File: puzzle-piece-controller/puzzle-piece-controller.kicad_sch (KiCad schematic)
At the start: 12 parts, among them J1 POGO PINS, J2 OUTPUT, J3 3.3V, J4 GND, J5 ANALOG, U1 MOUDLE-SEEEDUINO-XIAO-ESP32C3

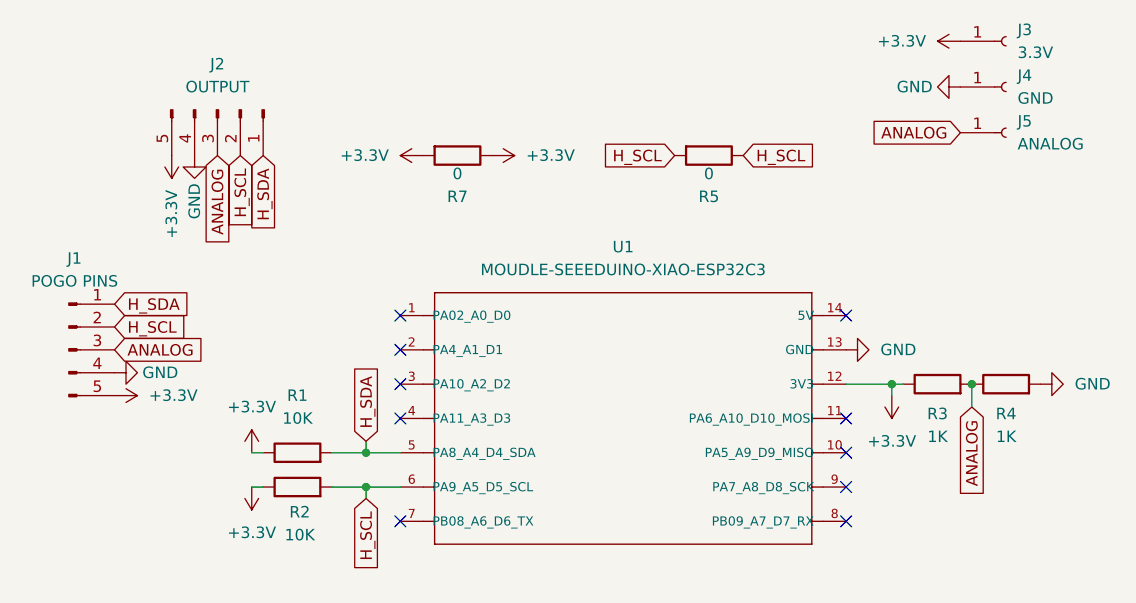
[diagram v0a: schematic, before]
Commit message: current puzzle with attiny and pogo pins
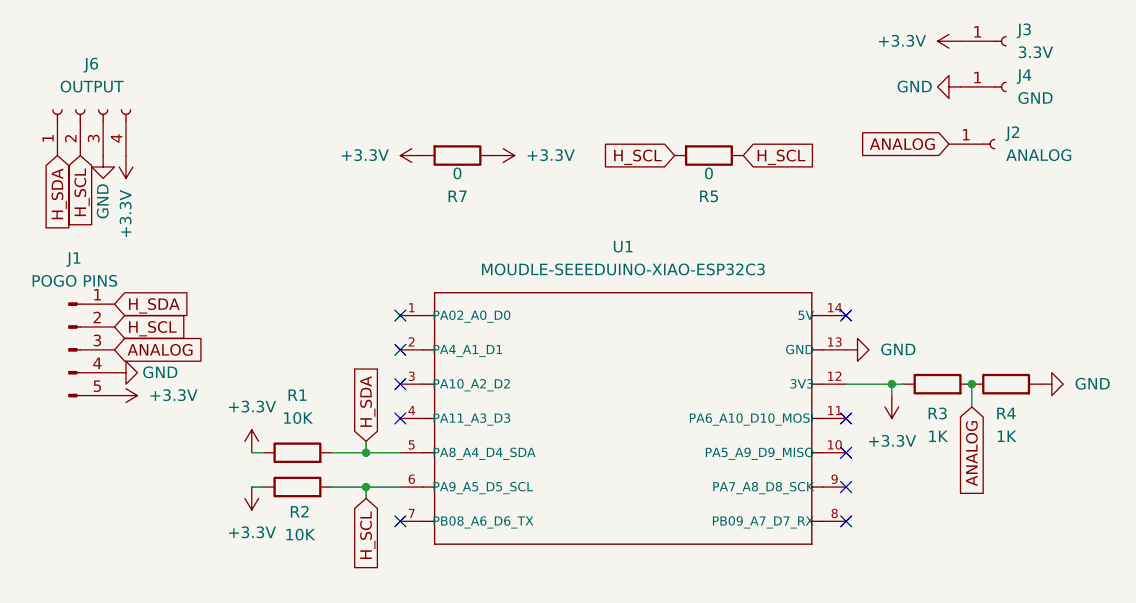
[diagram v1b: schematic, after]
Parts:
- removed J2: OUTPUT, Connector_PinHeader_2.54mm:PinHeader_1x05_P2.54mm_Vertical, symbol Connector:Conn_01x05_Pin
- removed J5: ANALOG, Connector_PinSocket_2.54mm:PinSocket_1x01_P2.54mm_Vertical, symbol Connector:Conn_01x01_Socket
- added J2: ANALOG, Connector_PinSocket_2.54mm:PinSocket_1x01_P2.54mm_Vertical, symbol Connector:Conn_01x01_Socket
- added J6: OUTPUT, Connector_PinSocket_2.54mm:PinSocket_1x04_P2.54mm_Vertical, symbol Connector:Conn_01x04_Socket
- U1: footprint xiao ESP32C3_PCB:MOUDLE14P-SMD-2.54-21X17.8MM -> fab:SeeedStudio_XIAO_ESP32C3
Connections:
- net +3.3V: now also J6.4 (Pin_4)
- net ANALOG: now also J2.1 (Pin_1)
- net GND: now also J6.3 (Pin_3)
- net H_SCL: now also J6.2 (Pin_2)
- net H_SDA: now also J6.1 (Pin_1)
